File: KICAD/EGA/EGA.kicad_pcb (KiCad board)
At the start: 2 copper layers, 39 parts, among them J1 12V, J10 TEST_TRIG, J2 HC-SR04, J3 LCD 20x4, J4 RTC, J5 TEST_PWM, J6 FAN_12V_PWM_3.3V, J7 UART, J8 TEST_RPM, J9 TEST_ECHO, SW1 PAGINA, SW2 RESET, U1 LM7805_TO220, U2 LM317_TO-220, U3 Pico

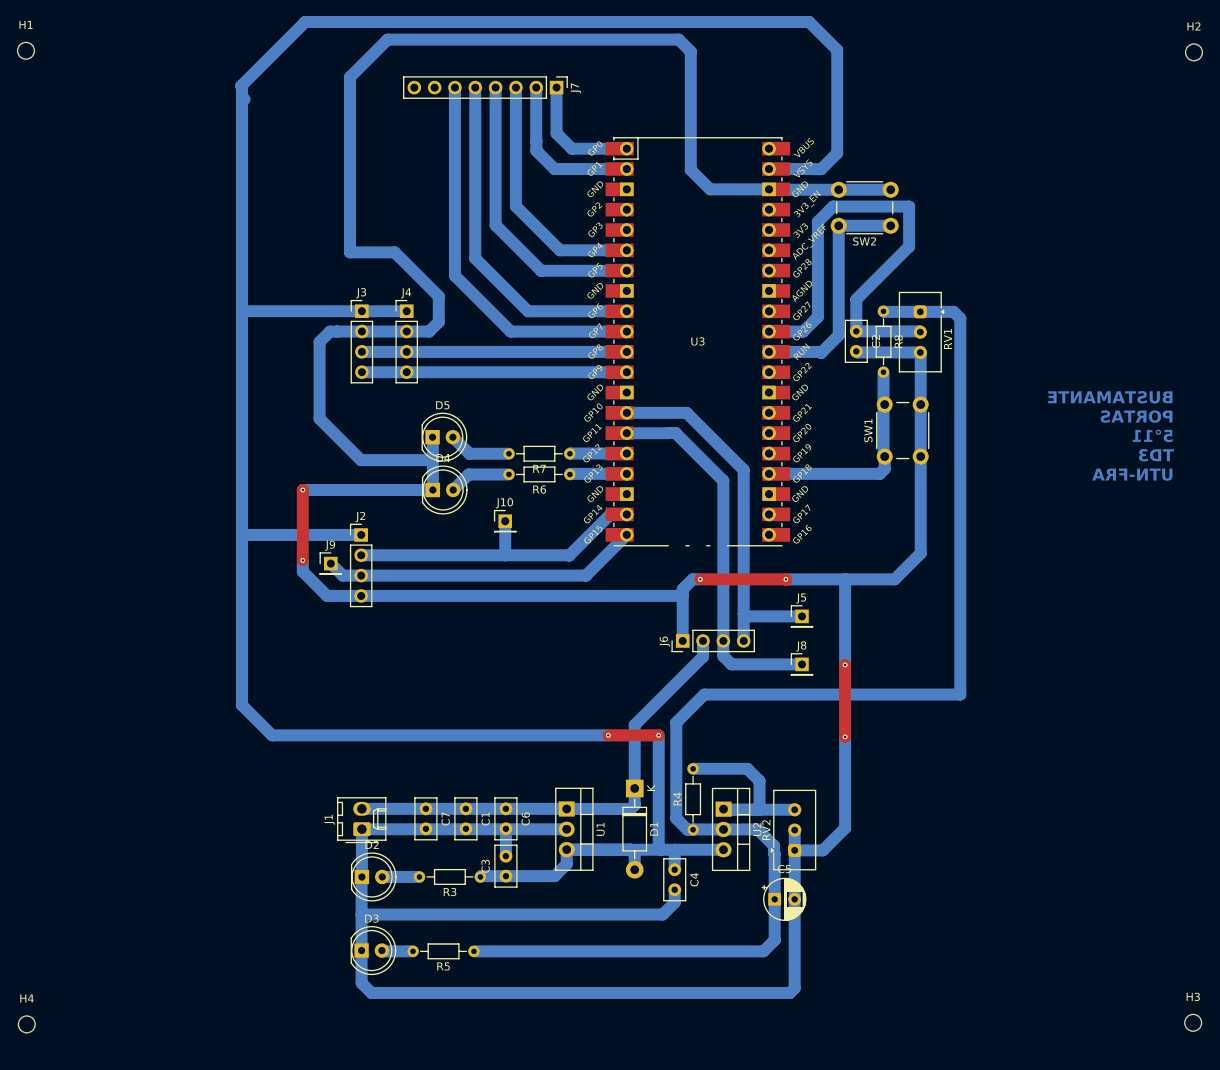
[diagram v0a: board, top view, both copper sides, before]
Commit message: Plano de masa en PCB
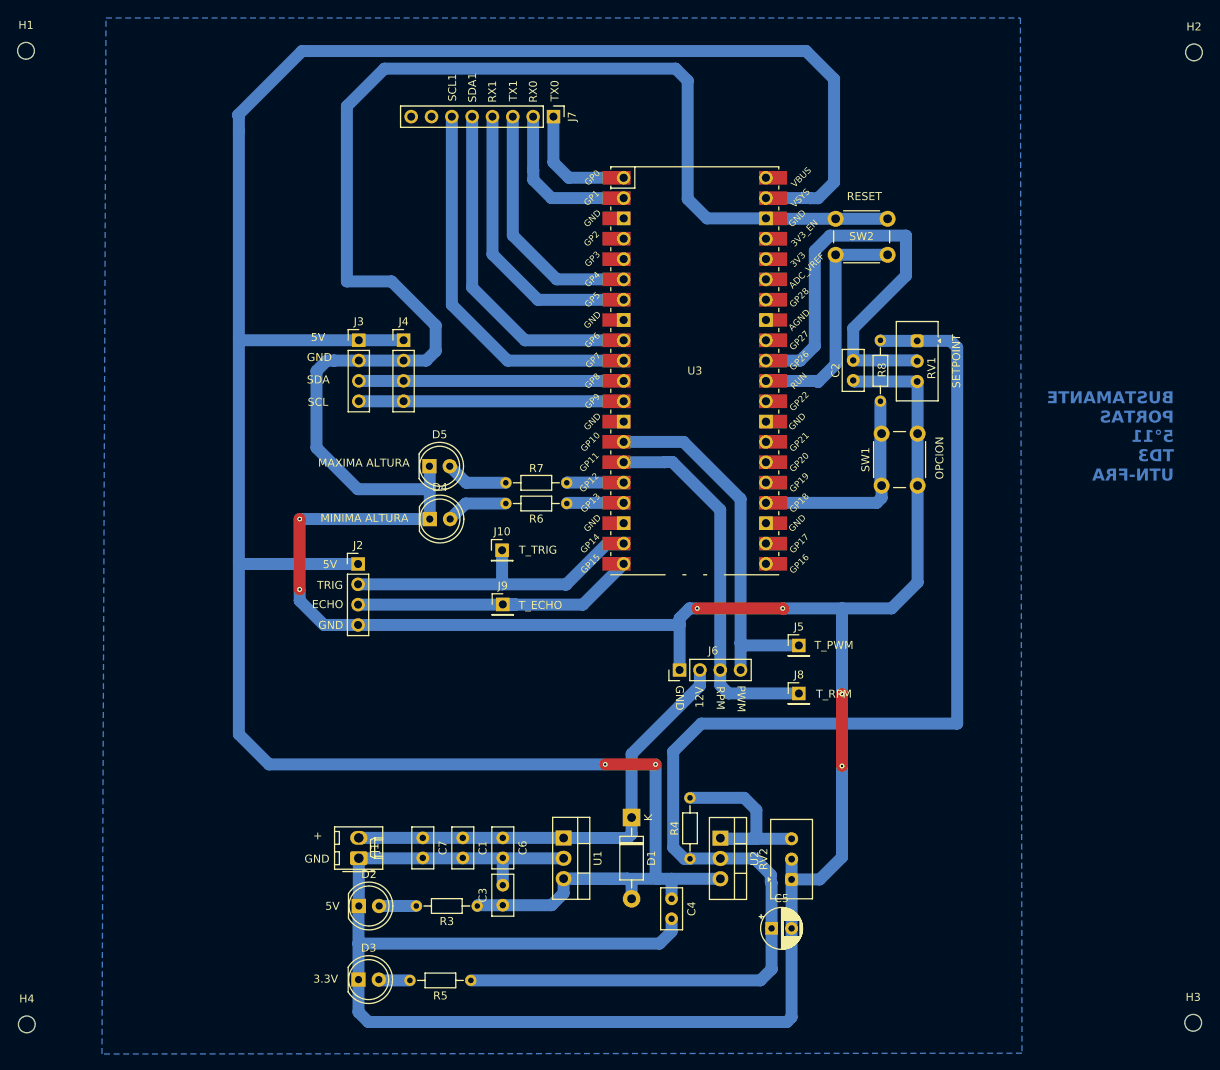
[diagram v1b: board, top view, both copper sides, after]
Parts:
- moved J9 22.1 mm to (102.9, 99.6)
- moved D2 3.65 mm to (84.9, 137.3)
- moved R3 3.65 mm to (99.7, 137.3)
- moved J5 3.65 mm to (139.9, 104.7)
- moved J8 3.65 mm to (139.9, 110.7)
- moved D4 3.65 mm to (93.8, 88.9)
- moved R4 3.65 mm to (126.3, 131.4)
- moved R7 3.65 mm to (110.9, 84.4)
- moved U1 3.65 mm to (110.5, 128.8)
- moved U3 3.65 mm to (126.9, 70.4)
- moved R8 3.65 mm to (150.1, 66.6)
- moved J7 3.65 mm to (109.2, 38.6)
- moved C2 3.65 mm to (146.7, 69.1)
- moved RV1 3.65 mm to (154.7, 66.7)
- moved U2 3.65 mm to (130.1, 128.8)
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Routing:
- net ECHO: track 39.8 -> 37.0 mm
- added copper zone on B.Cu, net GND
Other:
- board text added: "+"
- board text added: "12V"
- board text added: "3.3V"
- board text added: "5V"
- board text added: "ECHO"
- board text added: "GND"
- board text added: "MAXIMA ALTURA"
- board text added: "MINIMA ALTURA"
- board text added: "OPCION"
- board text added: "PWM"
- board text added: "RESET"
- board text added: "RPM"
- board text added: "RX0"
- board text added: "RX1"
- board text added: "SCL"
- board text added: "SCL1"
- board text added: "SDA"
- board text added: "SDA1"
- board text added: "SETPOINT"
- board text added: "TRIG"
- board text added: "TX0"
- board text added: "TX1"
- board text added: "T_ECHO"
- board text added: "T_PWM"
- board text added: "T_RPM"
- board text added: "T_TRIG"
